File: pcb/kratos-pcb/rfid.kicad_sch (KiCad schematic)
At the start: 1 part

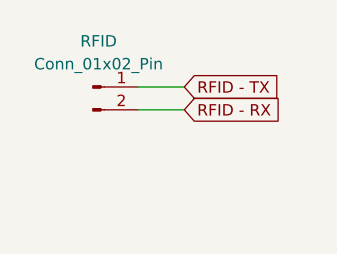
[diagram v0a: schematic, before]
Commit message: ### added
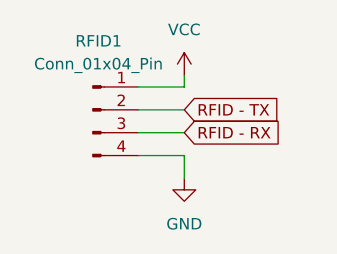
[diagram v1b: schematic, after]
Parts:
- removed RFID: Conn_01x02_Pin, symbol Connector:Conn_01x02_Pin
- added RFID1: Conn_01x04_Pin, Connector_PinHeader_2.00mm:PinHeader_1x04_P2.00mm_Vertical, symbol Connector:Conn_01x04_Pin
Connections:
- net RFID - RX: now also RFID1.3 (Pin_3)
- net RFID - TX: now also RFID1.2 (Pin_2)
- new net GND: RFID1.4 (Pin_4)
- new net VCC: RFID1.1 (Pin_1)
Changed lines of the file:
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@@
 (kicad_sch (version 20230121) (generator eeschema)
   (paper "A4")
+  (wire (pts (xy 100.33 99.06) (xy 105.41 99.06))
+    (stroke (width 0) (type default))
+  )
+  (wire (pts (xy 100.33 101.6) (xy 105.41 101.6))
+    (stroke (width 0) (type default))
+  )
+  (wire (pts (xy 100.33 104.14) (xy 105.41 104.14))
+    (stroke (width 0) (type default))
+  )
+  (wire (pts (xy 105.41 104.14) (xy 105.41 106.68))
+    (stroke (width 0) (type default))
+  )
   (wire (pts (xy 100.33 96.52) (xy 105.41 96.52))
     (stroke (width 0) (type default))
   )
-  (wire (pts (xy 100.33 99.06) (xy 105.41 99.06))
+  (wire (pts (xy 105.41 96.52) (xy 105.41 95.25))
     (stroke (width 0) (type default))
   )
-  (global_label "RFID - TX" (shape input) (at 105.41 96.52 0) (fields_autoplaced)
+  (global_label "RFID - RX" (shape input) (at 105.41 101.6 0) (fields_autoplaced)
     (effects (font (size 1.27 1.27)) (justify left))
-    (property "Intersheetrefs" "${INTERSHEET_REFS}" (at 118.3133 96.52 0)
+    (property "Intersheetrefs" "${INTERSHEET_REFS}" (at 118.6157 101.6 0)
       (effects (font (size 1.27 1.27)) (justify left) hide)
     )
   )
-  (global_label "RFID - RX" (shape input) (at 105.41 99.06 0) (fields_autoplaced)
+  (global_label "RFID - TX" (shape input) (at 105.41 99.06 0) (fields_autoplaced)
     (effects (font (size 1.27 1.27)) (justify left))
-    (property "Intersheetrefs" "${INTERSHEET_REFS}" (at 118.6157 99.06 0)
+    (property "Intersheetrefs" "${INTERSHEET_REFS}" (at 118.3133 99.06 0)
       (effects (font (size 1.27 1.27)) (justify left) hide)
     )
   )
-  (symbol (lib_id "Connector:Conn_01x02_Pin") (at 95.25 96.52 0) (unit 1)
+  (symbol (lib_id "power:GND") (at 105.41 106.68 0) (unit 1)
     (in_bom yes) (on_board yes) (dnp no) (fields_autoplaced)
-    (property "Reference" "RFID" (at 95.885 91.44 0)
+    (property "Reference" "#PWR027" (at 105.41 113.03 0)
+      (effects (font (size 1.27 1.27)) hide)
+    )
+    (property "Value" "GND" (at 105.41 111.76 0)
       (effects (font (size 1.27 1.27)))
     )
-    (property "Value" "Conn_01x02_Pin" (at 95.885 93.98 0)
-      (effects (font (size 1.27 1.27)))
-    )
-    (property "Footprint" "" (at 95.25 96.52 0)
+    (property "Footprint" "" (at 105.41 106.68 0)
       (effects (font (size 1.27 1.27)) hide)
     )
-    (property "Datasheet" "~" (at 95.25 96.52 0)
+    (property "Datasheet" "" (at 105.41 106.68 0)
       (effects (font (size 1.27 1.27)) hide)
     )
-    (pin "2")
     (pin "1")
     (instances
       (project "kratos-pcb"
         (path "/12f1b997-8c5f-4ef7-b036-7873ddaba48e/7e83680a-c321-4d95-9d9a-9e6345d60e4b"
-          (reference "RFID") (unit 1)
+          (reference "#PWR027") (unit 1)
         )
       )
+    )
+  )
+  (symbol (lib_id "Connector:Conn_01x04_Pin") (at 95.25 99.06 0) (unit 1)
+    (in_bom yes) (on_board yes) (dnp no) (fields_autoplaced)
+    (property "Reference" "RFID1" (at 95.885 91.44 0)
+      (effects (font (size 1.27 1.27)))
+    )
+    (property "Value" "Conn_01x04_Pin" (at 95.885 93.98 0)
+      (effects (font (size 1.27 1.27)))
+    )
+    (property "Footprint" "Connector_PinHeader_2.00mm:PinHeader_1x04_P2.00mm_Vertical" (at 95.25 99.06 0)
+      (effects (font (size 1.27 1.27)) hide)
+    )
+    (property "Datasheet" "~" (at 95.25 99.06 0)
+      (effects (font (size 1.27 1.27)) hide)
+    )
+    (pin "1")
+    (pin "2")
+    (pin "3")
+    (pin "4")
+    (instances
+      (project "kratos-pcb"
+        (path "/12f1b997-8c5f-4ef7-b036-7873ddaba48e/7e83680a-c321-4d95-9d9a-9e6345d60e4b"
+          (reference "RFID1") (unit 1)
+        )
+      )
+    )
+  )
+  (symbol (lib_id "power:VCC") (at 105.41 95.25 0) (unit 1)
+    (in_bom yes) (on_board yes) (dnp no) (fields_autoplaced)
+    (property "Reference" "#PWR028" (at 105.41 99.06 0)
+      (effects (font (size 1.27 1.27)) hide)
+    )
+    (property "Value" "VCC" (at 105.41 90.17 0)
+      (effects (font (size 1.27 1.27)))
+    )
+    (property "Footprint" "" (at 105.41 95.25 0)
+      (effects (font (size 1.27 1.27)) hide)
+    )
+    (property "Datasheet" "" (at 105.41 95.25 0)
+      (effects (font (size 1.27 1.27)) hide)
+    )
+    (pin "1")
+    (instances
+      (project "kratos-pcb"
+        (path "/12f1b997-8c5f-4ef7-b036-7873ddaba48e/7e83680a-c321-4d95-9d9a-9e6345d60e4b"
+          (reference "#PWR028") (unit 1)
+        )
+      )

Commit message: ### added
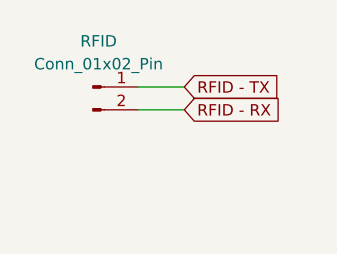
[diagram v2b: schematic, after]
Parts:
- removed RFID1: Conn_01x04_Pin, Connector_PinHeader_2.00mm:PinHeader_1x04_P2.00mm_Vertical, symbol Connector:Conn_01x04_Pin
- added RFID: Conn_01x02_Pin, symbol Connector:Conn_01x02_Pin
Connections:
- net RFID - RX: now also RFID.2 (Pin_2)
- net RFID - TX: now also RFID.1 (Pin_1)
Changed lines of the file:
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@@
 (kicad_sch (version 20230121) (generator eeschema)
   (paper "A4")
+  (wire (pts (xy 100.33 96.52) (xy 105.41 96.52))
+    (stroke (width 0) (type default))
+  )
   (wire (pts (xy 100.33 99.06) (xy 105.41 99.06))
     (stroke (width 0) (type default))
   )
-  (wire (pts (xy 100.33 101.6) (xy 105.41 101.6))
-    (stroke (width 0) (type default))
-  )
-  (wire (pts (xy 100.33 104.14) (xy 105.41 104.14))
-    (stroke (width 0) (type default))
-  )
-  (wire (pts (xy 105.41 104.14) (xy 105.41 106.68))
-    (stroke (width 0) (type default))
-  )
-  (wire (pts (xy 100.33 96.52) (xy 105.41 96.52))
-    (stroke (width 0) (type default))
-  )
-  (wire (pts (xy 105.41 96.52) (xy 105.41 95.25))
-    (stroke (width 0) (type default))
-  )
-  (global_label "RFID - RX" (shape input) (at 105.41 101.6 0) (fields_autoplaced)
+  (global_label "RFID - TX" (shape input) (at 105.41 96.52 0) (fields_autoplaced)
     (effects (font (size 1.27 1.27)) (justify left))
-    (property "Intersheetrefs" "${INTERSHEET_REFS}" (at 118.6157 101.6 0)
+    (property "Intersheetrefs" "${INTERSHEET_REFS}" (at 118.3133 96.52 0)
       (effects (font (size 1.27 1.27)) (justify left) hide)
     )
   )
-  (global_label "RFID - TX" (shape input) (at 105.41 99.06 0) (fields_autoplaced)
+  (global_label "RFID - RX" (shape input) (at 105.41 99.06 0) (fields_autoplaced)
     (effects (font (size 1.27 1.27)) (justify left))
-    (property "Intersheetrefs" "${INTERSHEET_REFS}" (at 118.3133 99.06 0)
+    (property "Intersheetrefs" "${INTERSHEET_REFS}" (at 118.6157 99.06 0)
       (effects (font (size 1.27 1.27)) (justify left) hide)
     )
   )
-  (symbol (lib_id "power:GND") (at 105.41 106.68 0) (unit 1)
+  (symbol (lib_id "Connector:Conn_01x02_Pin") (at 95.25 96.52 0) (unit 1)
     (in_bom yes) (on_board yes) (dnp no) (fields_autoplaced)
-    (property "Reference" "#PWR027" (at 105.41 113.03 0)
+    (property "Reference" "RFID" (at 95.885 91.44 0)
+      (effects (font (size 1.27 1.27)))
+    )
+    (property "Value" "Conn_01x02_Pin" (at 95.885 93.98 0)
+      (effects (font (size 1.27 1.27)))
+    )
+    (property "Footprint" "" (at 95.25 96.52 0)
       (effects (font (size 1.27 1.27)) hide)
     )
-    (property "Value" "GND" (at 105.41 111.76 0)
-      (effects (font (size 1.27 1.27)))
-    )
-    (property "Footprint" "" (at 105.41 106.68 0)
+    (property "Datasheet" "~" (at 95.25 96.52 0)
       (effects (font (size 1.27 1.27)) hide)
     )
-    (property "Datasheet" "" (at 105.41 106.68 0)
-      (effects (font (size 1.27 1.27)) hide)
-    )
+    (pin "2")
     (pin "1")
     (instances
       (project "kratos-pcb"
         (path "/12f1b997-8c5f-4ef7-b036-7873ddaba48e/7e83680a-c321-4d95-9d9a-9e6345d60e4b"
-          (reference "#PWR027") (unit 1)
+          (reference "RFID") (unit 1)
         )
       )
-    )
-  )
-  (symbol (lib_id "Connector:Conn_01x04_Pin") (at 95.25 99.06 0) (unit 1)
-    (in_bom yes) (on_board yes) (dnp no) (fields_autoplaced)
-    (property "Reference" "RFID1" (at 95.885 91.44 0)
-      (effects (font (size 1.27 1.27)))
-    )
-    (property "Value" "Conn_01x04_Pin" (at 95.885 93.98 0)
-      (effects (font (size 1.27 1.27)))
-    )
-    (property "Footprint" "Connector_PinHeader_2.00mm:PinHeader_1x04_P2.00mm_Vertical" (at 95.25 99.06 0)
-      (effects (font (size 1.27 1.27)) hide)
-    )
-    (property "Datasheet" "~" (at 95.25 99.06 0)
-      (effects (font (size 1.27 1.27)) hide)
-    )
-    (pin "1")
-    (pin "2")
-    (pin "3")
-    (pin "4")
-    (instances
-      (project "kratos-pcb"
-        (path "/12f1b997-8c5f-4ef7-b036-7873ddaba48e/7e83680a-c321-4d95-9d9a-9e6345d60e4b"
-          (reference "RFID1") (unit 1)
-        )
-      )
-    )
-  )
-  (symbol (lib_id "power:VCC") (at 105.41 95.25 0) (unit 1)
-    (in_bom yes) (on_board yes) (dnp no) (fields_autoplaced)
-    (property "Reference" "#PWR028" (at 105.41 99.06 0)
-      (effects (font (size 1.27 1.27)) hide)
-    )
-    (property "Value" "VCC" (at 105.41 90.17 0)
-      (effects (font (size 1.27 1.27)))
-    )
-    (property "Footprint" "" (at 105.41 95.25 0)
-      (effects (font (size 1.27 1.27)) hide)
-    )
-    (property "Datasheet" "" (at 105.41 95.25 0)
-      (effects (font (size 1.27 1.27)) hide)
-    )
-    (pin "1")
-    (instances
-      (project "kratos-pcb"
-        (path "/12f1b997-8c5f-4ef7-b036-7873ddaba48e/7e83680a-c321-4d95-9d9a-9e6345d60e4b"
-          (reference "#PWR028") (unit 1)
-        )
-      )
